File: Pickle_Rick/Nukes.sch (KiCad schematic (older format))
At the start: 21 parts, among them J6 Screw_Terminal_01x02, J7 Screw_Terminal_01x02, J8 Screw_Terminal_01x02, Q4 PMV20ENR, Q5 PMV20ENR, U10 LTV-817S, U9 LTV-817S

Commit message: updated optocoupler, usb kinda weird atm ¯\_(ツ)_/¯
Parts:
- removed U10, U9: LTV-817S, Package_DIP:SMDIP-4_W9.53mm, symbol Isolator:LTV-817S
- added U? (x2): LTV-354T, Package_SO:SO-4_4.4x3.6mm_P2.54mm, symbol Isolator:LTV-354T
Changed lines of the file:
@@
 Wire Wire Line
 	8600 4150 8600 4200
-$Comp
-L Isolator:LTV-817S U?
-U 1 1 5DE04B23
-P 9450 4700
-AR Path="/5DDE6CFA/5DE04B23" Ref="U?"  Part="1"
-AR Path="/5DDE1103/5DE04B23" Ref="U10"  Part="1"
-F 0 "U10" H 9450 5025 50  0000 C CNN
-F 1 "LTV-817S" H 9450 4934 50  0000 C CNN
-F 2 "Package_DIP:SMDIP-4_W9.53mm" H 9450 4400 50  0001 C CNN
-F 3 "http://www.us.liteon.com/downloads/LTV-817-827-847.PDF" H 9100 5000 50  0001 C CNN
-	1    9450 4700
-	-1   0    0    -1
-$EndComp
 Wire Wire Line
 	9750 4150 9750 4600
@@
 Wire Wire Line
 	4350 4300 4350 4350
-$Comp
-L Isolator:LTV-817S U?
-U 1 1 5DE32360
-P 5200 4850
-AR Path="/5DDE6CFA/5DE32360" Ref="U?"  Part="1"
-AR Path="/5DDE1103/5DE32360" Ref="U9"  Part="1"
-F 0 "U9" H 5200 5175 50  0000 C CNN
-F 1 "LTV-817S" H 5200 5084 50  0000 C CNN
-F 2 "Package_DIP:SMDIP-4_W9.53mm" H 5200 4550 50  0001 C CNN
-F 3 "http://www.us.liteon.com/downloads/LTV-817-827-847.PDF" H 4850 5150 50  0001 C CNN
-	1    5200 4850
-	-1   0    0    -1
-$EndComp
 Wire Wire Line
 	5500 4300 5500 4750
@@
 Wire Wire Line
 	5450 2600 6350 2600
+$Comp
+L Isolator:LTV-354T U?
+U 1 1 603DC15B
+P 5200 4850
+F 0 "U?" H 5200 5175 50  0000 C CNN
+F 1 "LTV-354T" H 5200 5084 50  0000 C CNN
+F 2 "Package_SO:SO-4_4.4x3.6mm_P2.54mm" H 5000 4650 50  0001 L CIN
+F 3 "http://optoelectronics.liteon.com/upload/download/DS70-2001-004/S_110_LTV-354T%2020140520.pdf" H 5225 4850 50  0001 L CNN
+	1    5200 4850
+	1    0    0    -1
+$EndComp
+$Comp
+L Isolator:LTV-354T U?
+U 1 1 603EA371
+P 9450 4700
+F 0 "U?" H 9450 5025 50  0000 C CNN
+F 1 "LTV-354T" H 9450 4934 50  0000 C CNN
+F 2 "Package_SO:SO-4_4.4x3.6mm_P2.54mm" H 9250 4500 50  0001 L CIN
+F 3 "http://optoelectronics.liteon.com/upload/download/DS70-2001-004/S_110_LTV-354T%2020140520.pdf" H 9475 4700 50  0001 L CNN
+	1    9450 4700
+	1    0    0    -1
+$EndComp
 $EndSCHEMATC

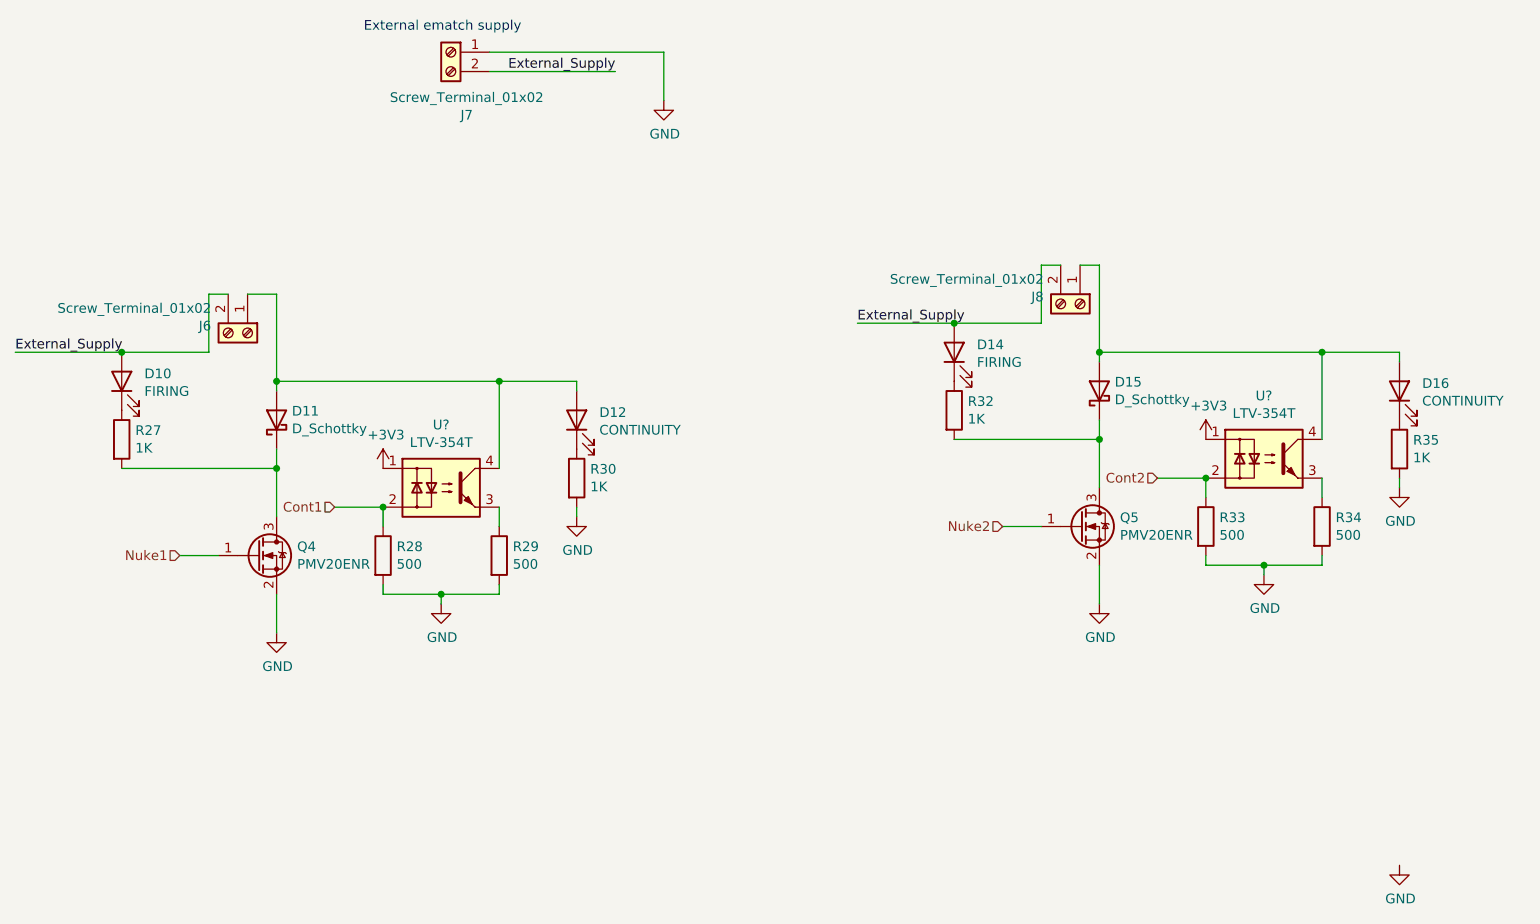
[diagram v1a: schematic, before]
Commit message: 50/50 that the usb will work
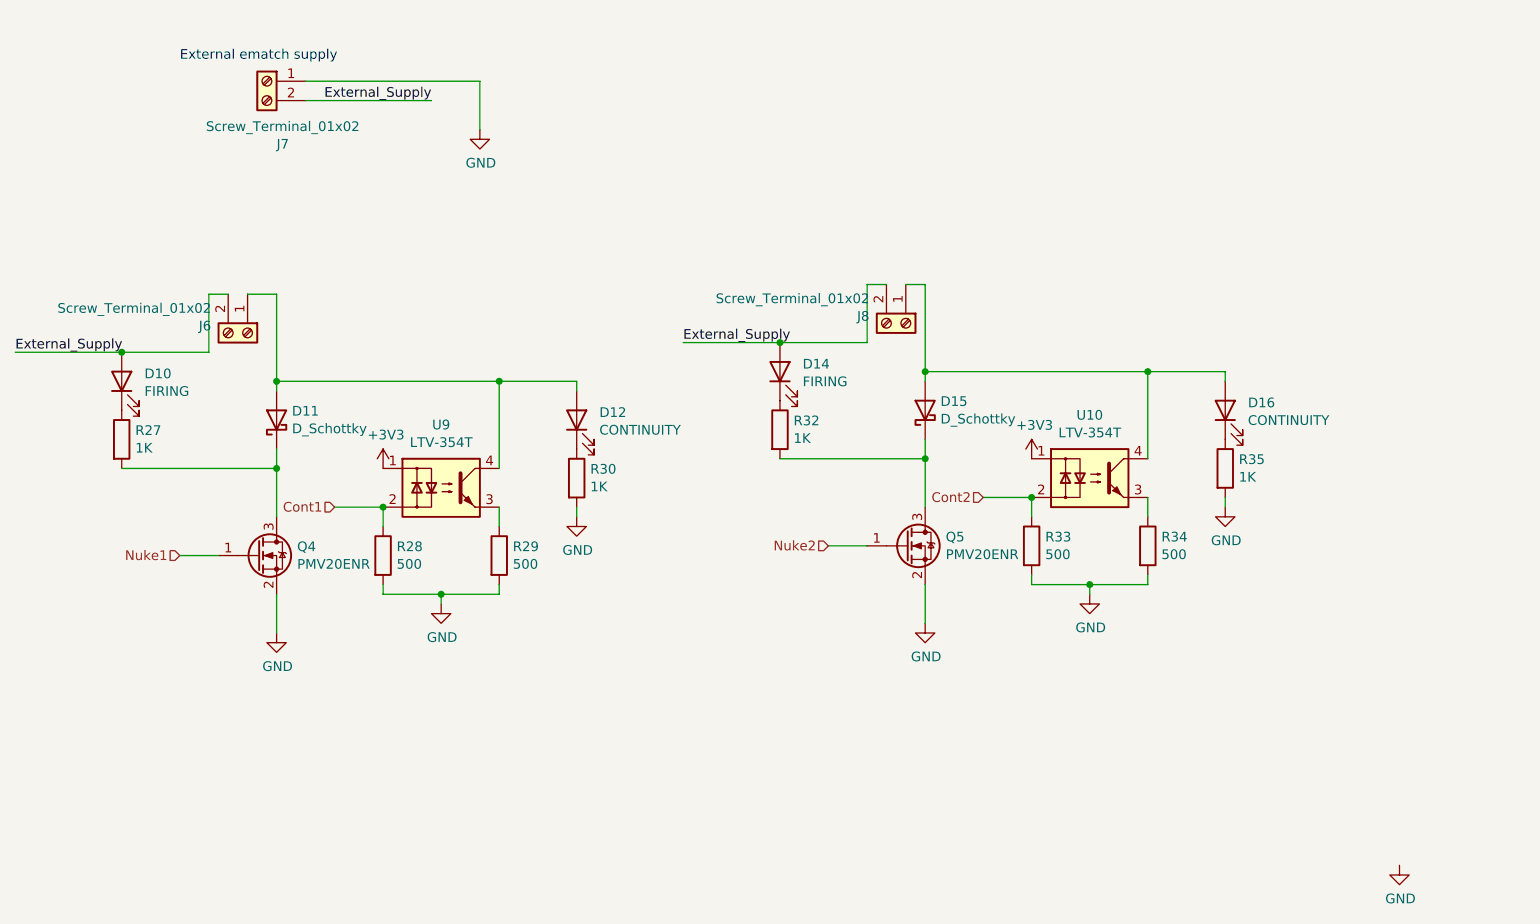
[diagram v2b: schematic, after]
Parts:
- gave numbers to parts that had none: 2
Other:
- moved on the sheet: D14, D15, D16, J7, J8, Q5, R32, R33, R34, R35, U10
